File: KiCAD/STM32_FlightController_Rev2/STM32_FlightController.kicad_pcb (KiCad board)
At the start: 4 copper layers, 42 x 44.4 mm, 56 parts, among them J1 629105150521, J2 JST_SH_SM08B-SRSS-TB_1x08-1MP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, J3 JST_SH_SM04B-SRSS-TB_1x04-1MP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, J4 JST_SH_SM04B-SRSS-TB_1x04-1MP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, J5 Conn_02x05_Odd_Even, SW1 PTS815SJM250SMTRLFS, SW2 PCM12SMTR, U1 SN74LVC1T45DBV, U2 ICM-20948, U3 STM32F405RGTx, U4 USBLC6-2SC6, U5 AMS1117-3.3, U6 TLV70018, U7 BMP390L, U8 SN74LVC1T45DBV, Y1 X32258MOB4SI

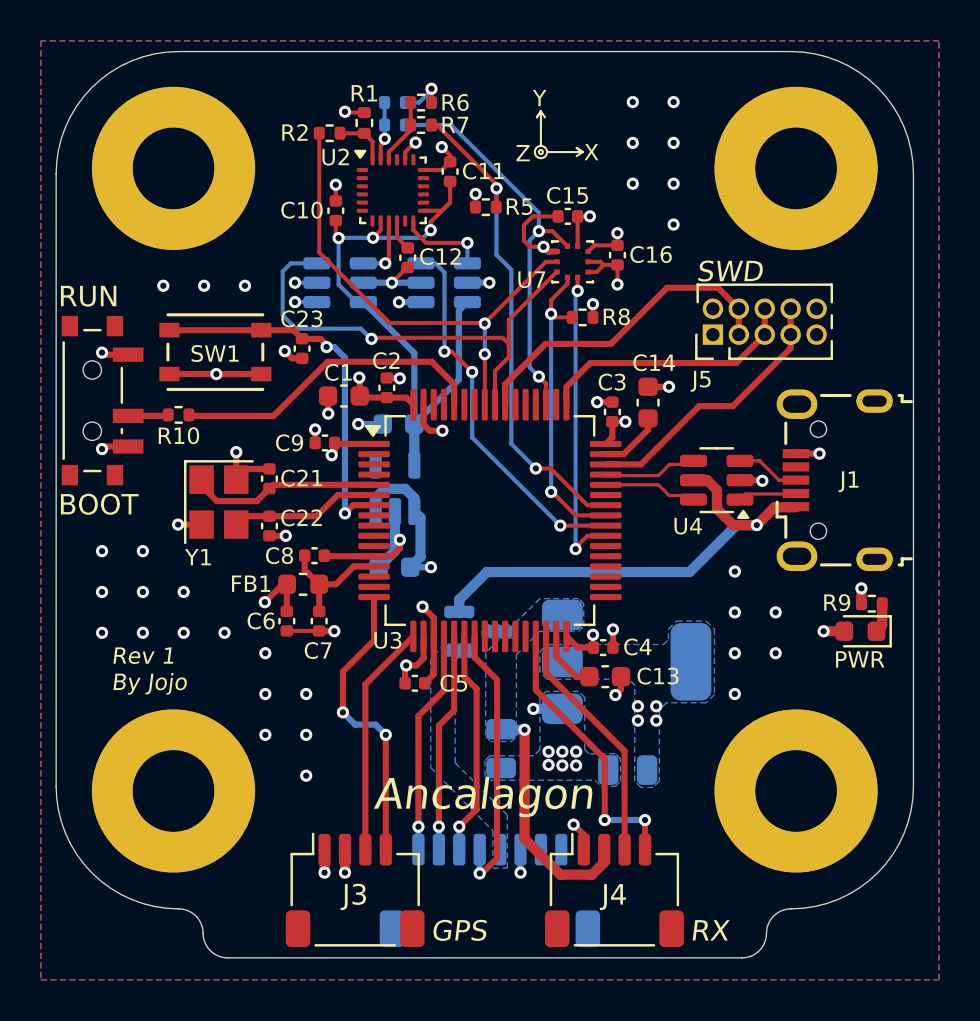
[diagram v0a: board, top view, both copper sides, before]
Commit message: aesthetics changes
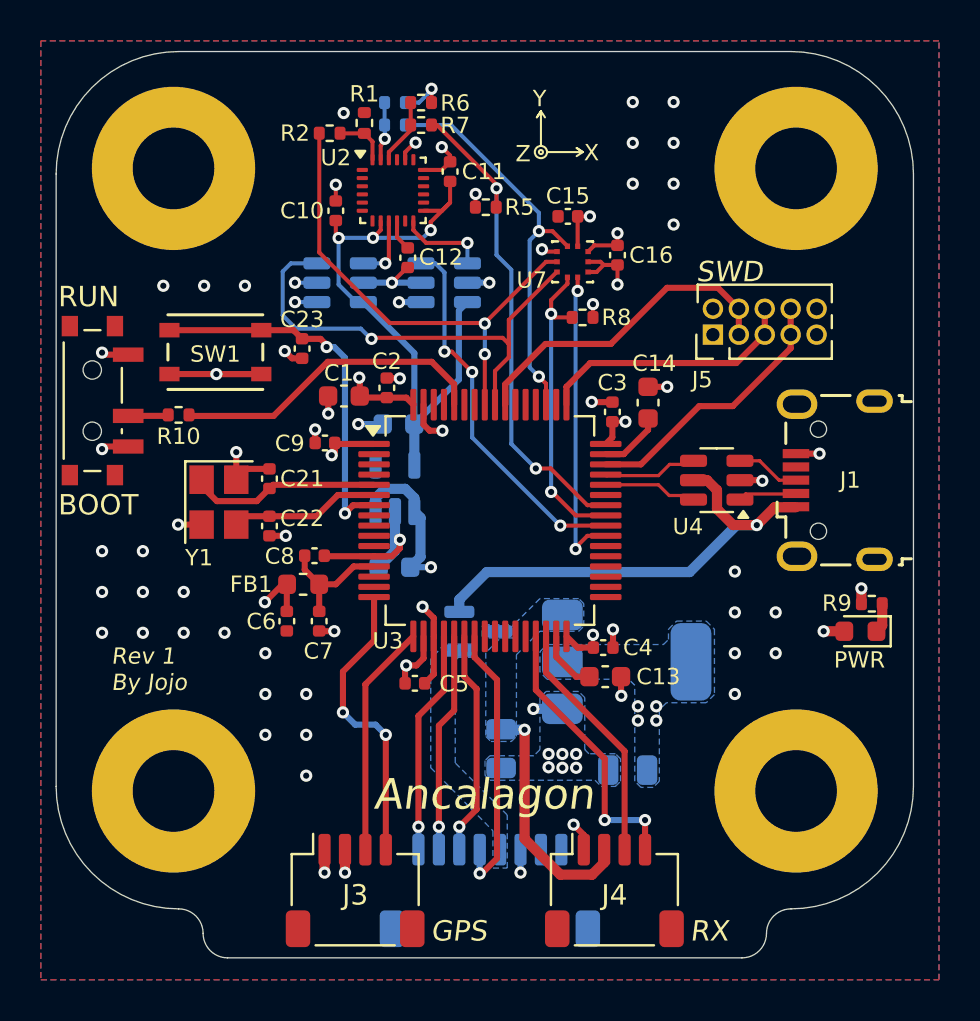
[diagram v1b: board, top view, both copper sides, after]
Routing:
- net GND: track 65.4 -> 59.3 mm
